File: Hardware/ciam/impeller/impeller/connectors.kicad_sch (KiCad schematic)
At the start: 15 parts, among them J12 Micro-Fit_2x2P, J29 USB_A, J4 MicroFit_2x2, J4 Pinheader_2x5, U19 TLP521-2, U2 B0503S-1WR3, U4 USBLC6-2SC6

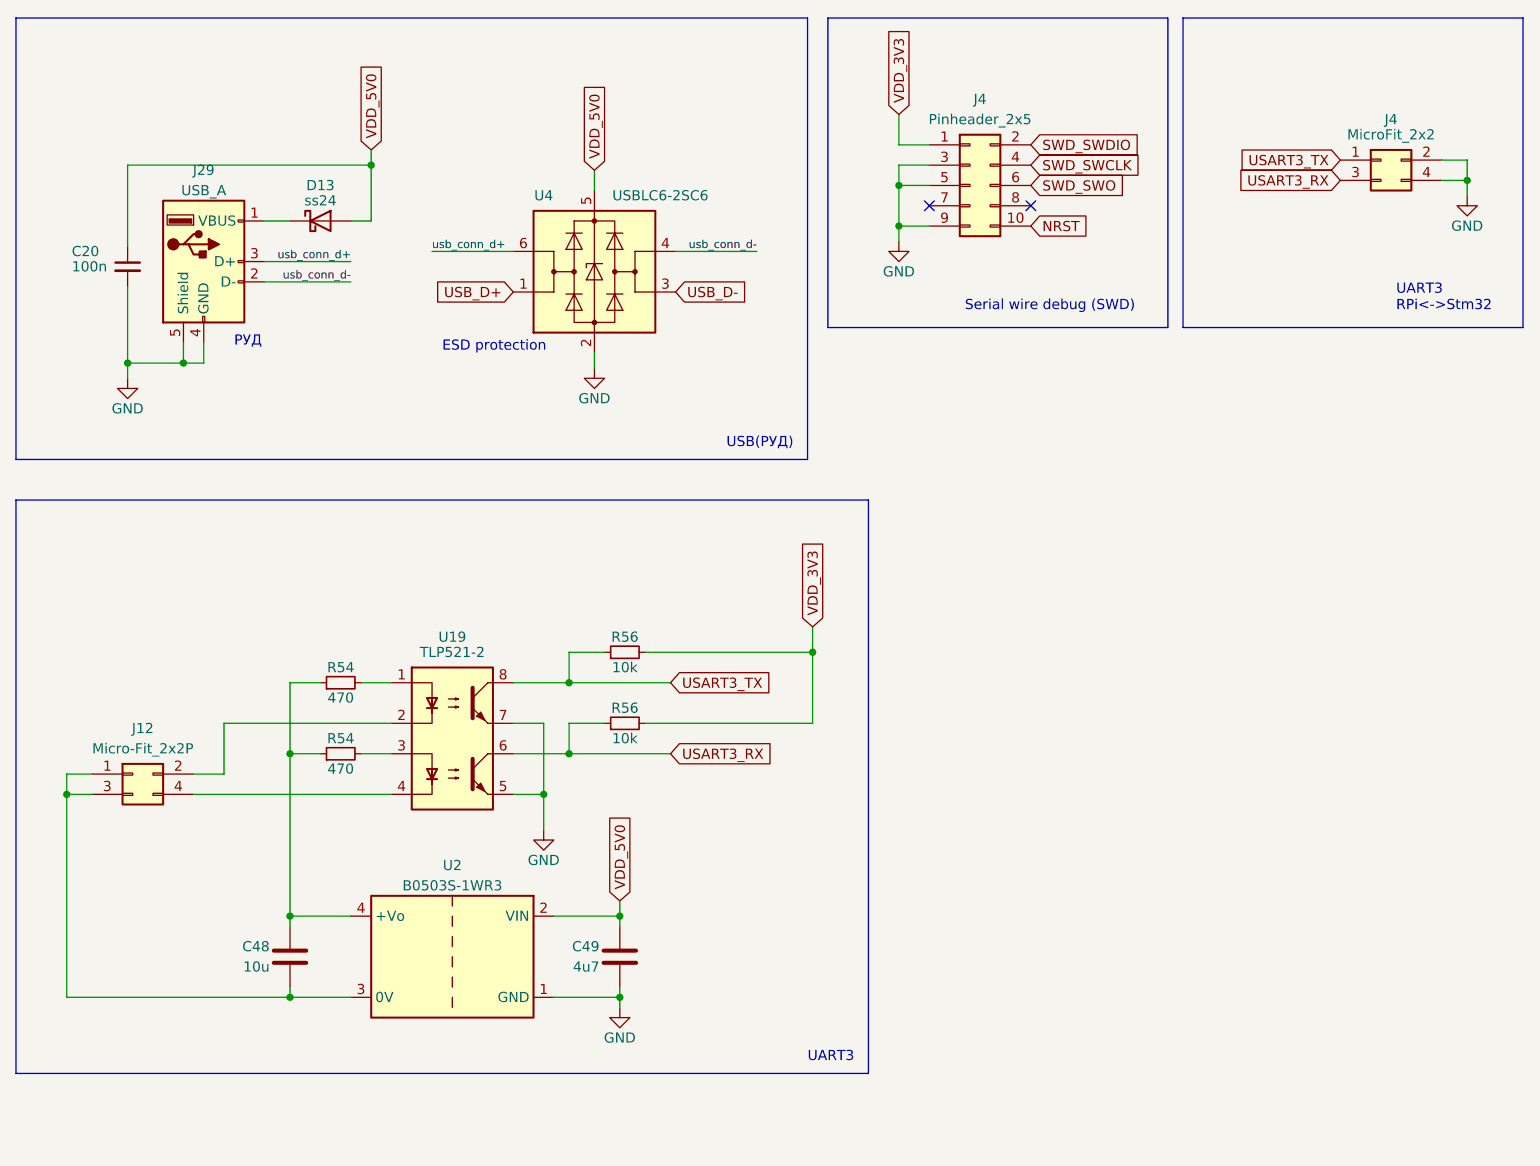
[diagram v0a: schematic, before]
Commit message: updated impeller project
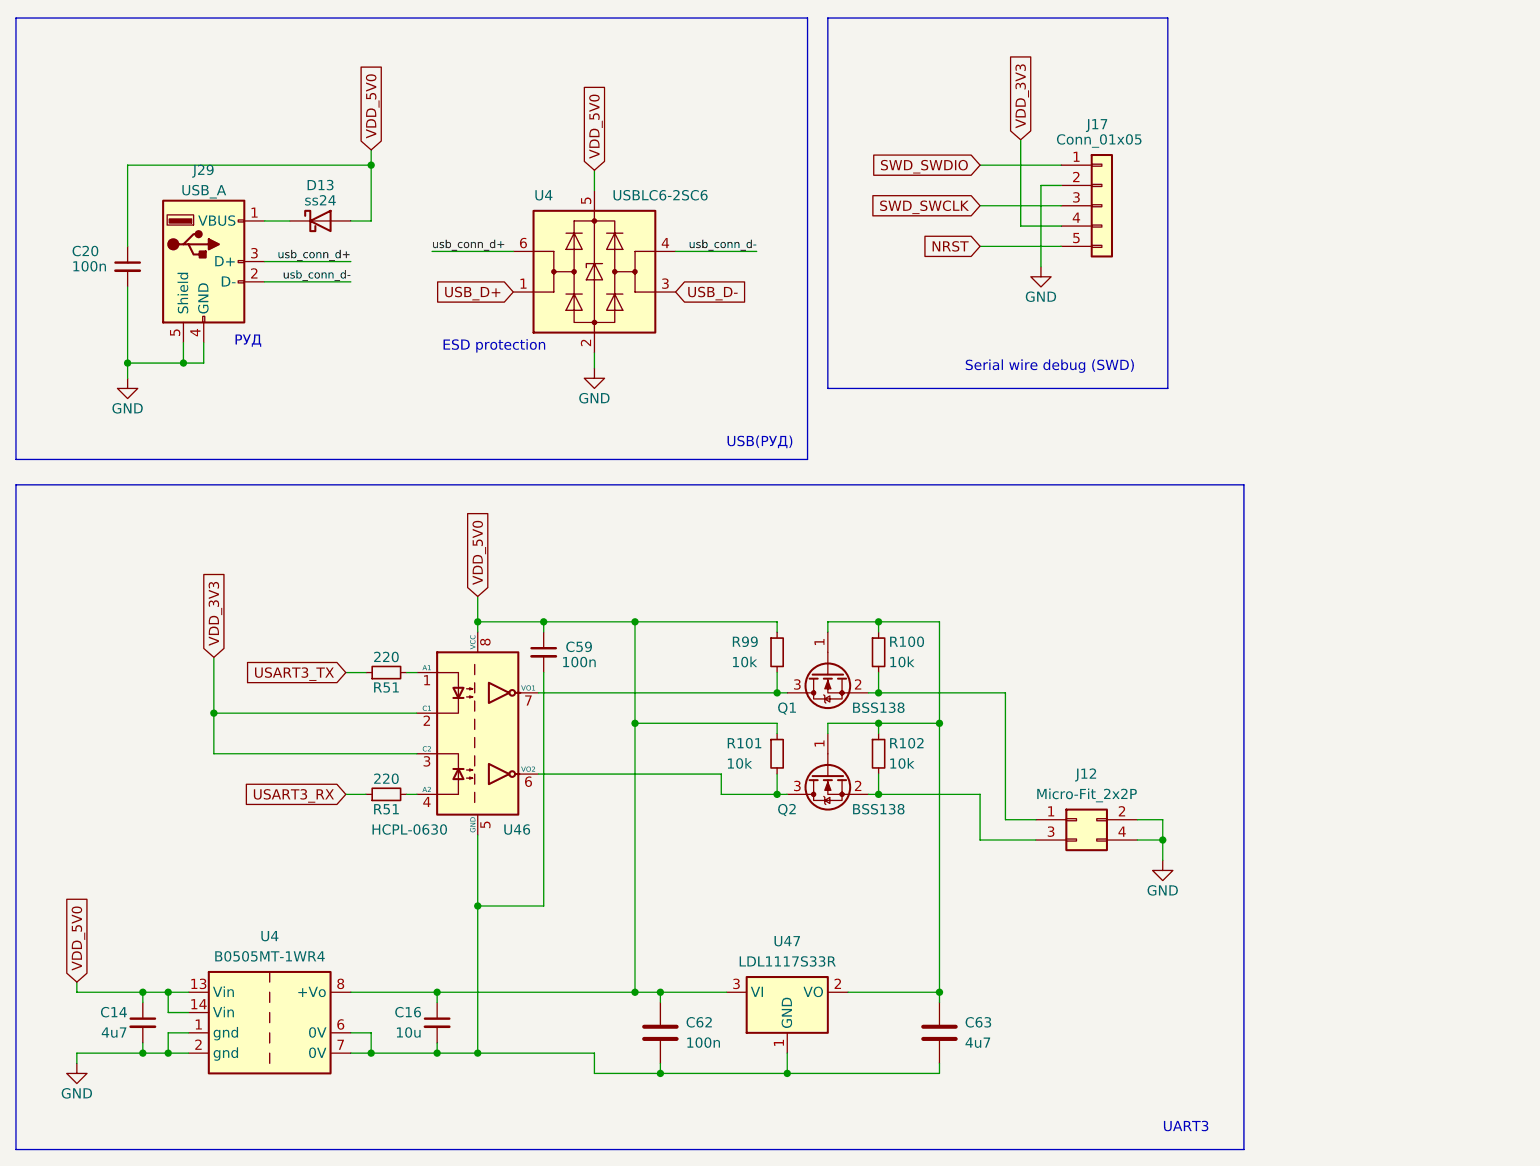
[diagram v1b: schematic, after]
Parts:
- removed C48: 10u, symbol Device:C
- removed C49: 4u7, symbol Device:C
- removed J4: Pinheader_2x5, Connector_PinHeader_1.27mm:PinHeader_2x05_P1.27mm_Vertical, symbol Connector_Generic:Conn_02x05_Odd_Even
- removed J4: MicroFit_2x2, symbol Connector_Generic:Conn_02x02_Odd_Even
- removed R54 (x2): 470, symbol Device:R_Small
- removed R56 (x2): 10k, symbol Device:R_Small
- removed U19: TLP521-2, symbol Isolator:TLP291
- removed U2: B0503S-1WR3, symbol Converter_DCDC:TMR-1211
- added C14: 4u7, symbol Device:C_Small
- added C16: 10u, symbol Device:C_Small
- added C59: 100n, symbol Device:C_Small
- added C62: 100n, symbol Device:C
- added C63: 4u7, symbol Device:C
- added J17: Conn_01x05, symbol Connector_Generic:Conn_01x05
- added Q1, Q2: BSS138, Package_TO_SOT_SMD:SOT-23, symbol Transistor_FET:BSS138
- added R100, R101, R102, R99: 10k, symbol Device:R_Small
- added R51 (x2): 220, symbol Device:R_Small
- added U4: B0505MT-1WR4, symbol Interface_CAN_LIN:ISO1050DUB
- added U46: HCPL-0630, Package_SO:SOIC-8_3.9x4.9mm_P1.27mm, symbol Isolator:HCPL-0630
- added U47: LDL1117S33R, Package_TO_SOT_SMD:SOT-223-3_TabPin2, symbol Regulator_Linear:LD1117S33TR_SOT223
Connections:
- net GND: now also J12.2 (Pin_2), J12.4 (Pin_4), C14.2, J17.2 (Pin_2), U4.1 (gnd), U4.2 (gnd)
- net NRST: now also J17.5 (Pin_5)
- net SWD_SWCLK: now also J17.3 (Pin_3)
- net SWD_SWDIO: now also J17.1 (Pin_1)
- net USART3_RX: now also R51.1
- net USART3_TX: now also R51.1
- net VDD_3V3: now also J17.4 (Pin_4), U46.2 (C1), U46.3 (C2)
- net VDD_5V0: now also C14.1, C16.1, C59.1, C62.1, R101.1, R99.1, U4.13 (Vin), U4.14 (Vin), U4.8 (+Vo), U46.8 (VCC), U47.3 (VI)
- net at J12.3 (Pin_3): now also Q2.2 (S), R102.2; no longer J12.1 (Pin_1)
- new net: C16.2, C59.2, C62.2, C63.2, U4.6 (0V), U4.7 (0V), U46.5 (GND), U47.1 (GND)
- new net: R51.2, U46.4 (A2)
- new net: R51.2, U46.1 (A1)
- new net: Q2.3 (D), R101.2, U46.6 (VO2)
- new net: Q1.3 (D), R99.2, U46.7 (VO1)
- new net: C63.1, Q1.1 (G), Q2.1 (G), R100.1, R102.1, U47.2 (VO)
- new net: J12.1 (Pin_1), Q1.2 (S), R100.2
- no-connect marks 2 -> 0
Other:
- note removed: "UART3 RPi<->Stm32"
- moved on the sheet: J12
